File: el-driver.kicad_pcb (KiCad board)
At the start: 2 copper layers, 39 x 26 mm, 39 parts, among them J1 Conn_01x03, J2 Conn_01x02, Q1 SI3493DDV-T1-GE3, Q2 BSS138, Q3 BSS214NW, Q4 BSS214NW, T1 42XL003-RC, U1 NE555D

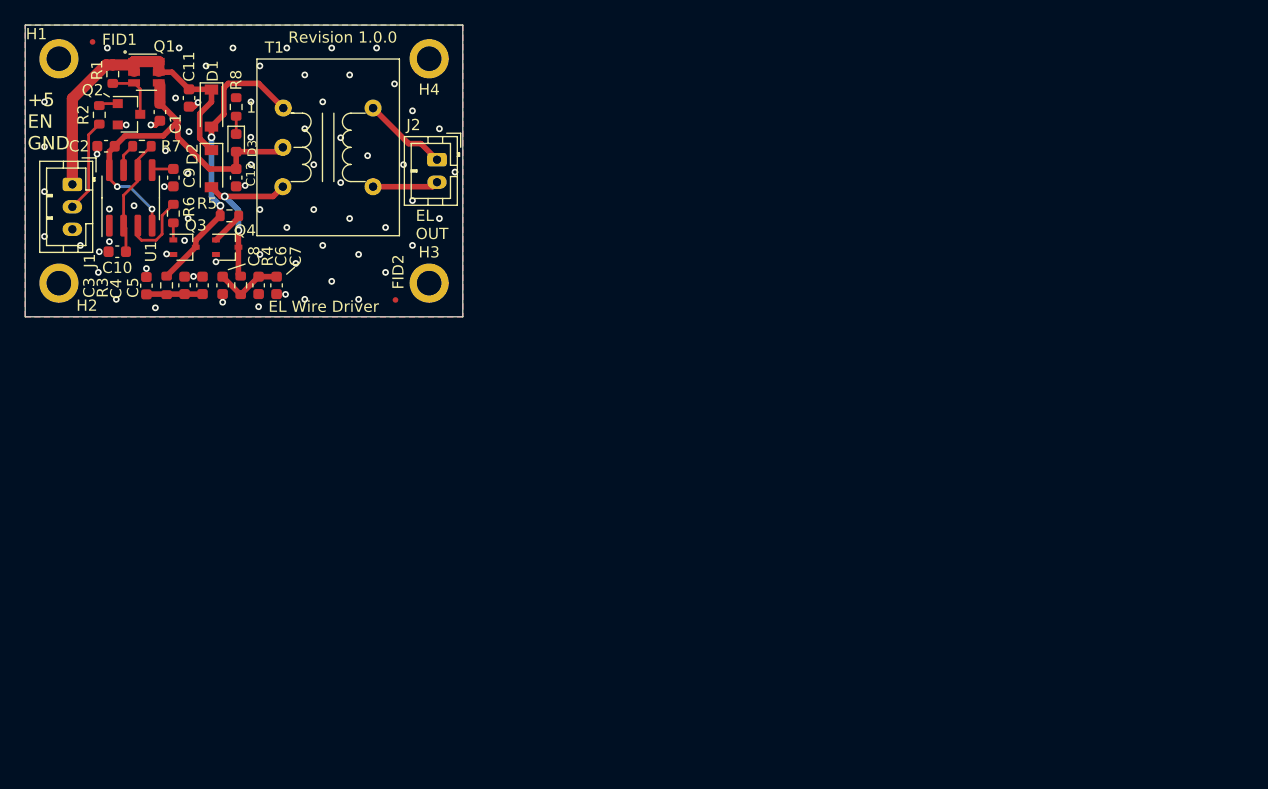
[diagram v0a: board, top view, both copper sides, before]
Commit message: Version 2.0.0
Signed-off-by: Aaron Williams <aaron.w2@gmail.com>
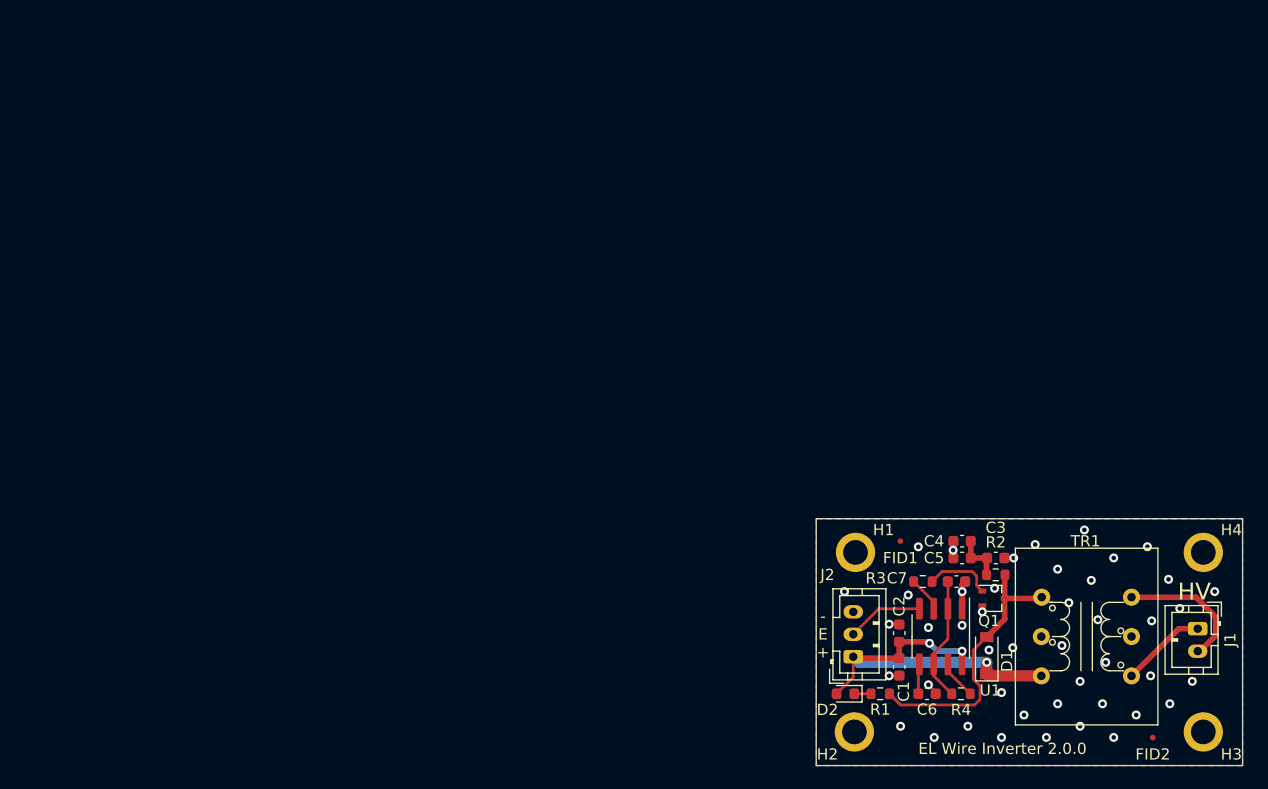
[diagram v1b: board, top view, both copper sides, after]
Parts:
- removed C10: 47nF, Capacitor_SMD:C_0603_1608Metric
- removed C11: 10uF, Capacitor_SMD:C_0603_1608Metric
- removed C12: 1uF, Capacitor_SMD:C_0603_1608Metric
- removed C8: 1nF, Capacitor_SMD:C_0603_1608Metric
- removed C9: 10nF, Capacitor_SMD:C_0603_1608Metric
- removed D3: LED, LED_SMD:LED_0603_1608Metric
- removed Q2: BSS138, Package_TO_SOT_SMD:SOT-23
- removed Q3, Q4: BSS214NW, Package_TO_SOT_SMD:SOT-323_SC-70
- removed R5, R6: 100k, Resistor_SMD:R_0603_1608Metric
- removed R7: 10k, Resistor_SMD:R_0603_1608Metric
- removed R8: 220, Resistor_SMD:R_0603_1608Metric
- removed the REF** at (114.3, 48.5)
- removed T1: 42XL003-RC, Aaron:Transformer_42XL_EI-14
- added REF**: OSHW-Logo2_7.3x6mm_SilkScreen, Symbol:OSHW-Logo2_7.3x6mm_SilkScreen, B.Cu at (194.1, 96.8)
- added TR1: Transformer-EI14, Aaron:Transformer_42XL_EI-14, F.Cu at (194.6, 88.5)
- C6: value 4.7nF -> 10nF
- C7: value 1nF -> 47nF
- D2: value SS24FL -> LED; footprint Diode_SMD:D_SOD-123 -> LED_SMD:LED_0603_1608Metric
- J1: value Conn_01x03 -> Conn_01x02; footprint Connector_JST:JST_PH_B3B-PH-K_1x03_P2.00mm_Vertical -> Connector_JST:JST_PH_B2B-PH-K_1x02_P2.00mm_Vertical
- J2: value Conn_01x02 -> Conn_01x03; footprint Connector_JST:JST_PH_B2B-PH-K_1x02_P2.00mm_Vertical -> Connector_JST:JST_PH_B3B-PH-K_1x03_P2.00mm_Vertical
- Q1: value SI3493DDV-T1-GE3 -> BSS214NW; footprint Package_TO_SOT_SMD:SOT-23-6 -> Package_TO_SOT_SMD:SOT-323_SC-70
- R1: value 100k -> 220
- R2: value 100k -> 39.2
- R3: value 39.2 -> 100k
- R4: value 39.2 -> 10k
- moved J1 107.8 mm to (204.5, 87.8)
- moved R2 89.8 mm to (186.5, 83.0), turned to 180 degrees
- moved Q1 88.9 mm to (186.3, 85.1)
- moved R1 87.9 mm to (176.2, 93.6), turned to 0 degrees
- moved REF** 87.3 mm to (182.4, 96.1)
- moved FID1 84.6 mm to (178.0, 80.0), turned to 180 degrees
- moved D1 84.6 mm to (185.7, 90.2), turned to 90 degrees
- moved H1 83.5 mm to (174.0, 81.0), turned to 180 degrees
- moved C2 83.0 mm to (177.9, 88.2), turned to 90 degrees
- moved C1 82.4 mm to (177.9, 91.2)
- moved U1 82.1 mm to (181.6, 88.5), turned to 270 degrees
- moved H4 81.8 mm to (205.0, 81.0), turned to 180 degrees
- moved H2 81.4 mm to (173.9, 97.0), turned to 180 degrees
- moved H3 79.8 mm to (205.0, 97.0), turned to 180 degrees
- moved C3 79.5 mm to (186.5, 81.5), turned to 0 degrees
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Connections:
- C1 pad 1: /5V_SW -> +5V
- C2 pad 1: /5V_SW -> +5V
- C7 pad 1: Net-(C6-Pad1) -> Net-(C7-Pad1)
- D2 pad 1: +5V -> Net-(D2-Pad1)
- D2 pad 2: Net-(D2-Pad2) -> +5V
- J1 pad 1: +5V -> Net-(J1-Pad1)
- J1 pad 2: /EN -> Net-(J1-Pad2)
- J2 pad 1: Net-(J2-Pad1) -> +5V
- J2 pad 2: Net-(J2-Pad2) -> /EN
- Q1 pad 1: +5V -> Net-(Q1-Pad1)
- Q1 pad 2: +5V -> GND
- Q1 pad 3: Net-(Q1-Pad3) -> Net-(D1-Pad2)
- R1 pad 1: +5V -> Net-(D2-Pad1)
- R1 pad 2: Net-(Q1-Pad3) -> Net-(D1-Pad2)
- R2 pad 1: /EN -> Net-(D1-Pad2)
- R2 pad 2: Net-(Q2-Pad1) -> Net-(C3-Pad1)
- R3 pad 1: Net-(D1-Pad2) -> Net-(R3-Pad1)
- R3 pad 2: Net-(C3-Pad1) -> Net-(Q1-Pad1)
- R4 pad 1: Net-(D2-Pad2) -> Net-(R4-Pad1)
- R4 pad 2: Net-(C6-Pad1) -> Net-(C7-Pad1)
- U1 pad 2: Net-(C10-Pad1) -> Net-(C7-Pad1)
- U1 pad 3: Net-(R6-Pad1) -> Net-(R3-Pad1)
- U1 pad 4: /5V_SW -> /EN
- U1 pad 5: Net-(C9-Pad1) -> Net-(C6-Pad1)
- U1 pad 6: Net-(C10-Pad1) -> Net-(C7-Pad1)
- U1 pad 7: Net-(R7-Pad1) -> Net-(R4-Pad1)
- U1 pad 8: /5V_SW -> +5V
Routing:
- net /5V_SW: track 33.6 -> 0.00 mm, vias 2 -> 0
- net Net-(D2-Pad2): track 14.8 -> 0.00 mm, vias 2 -> 0
- net Net-(J1-Pad2): track 0.00 -> 12.1 mm
- net Net-(C7-Pad1): track 0.00 -> 11.2 mm
- net Net-(C10-Pad1): track 10.5 -> 0.00 mm
- net Net-(J1-Pad1): track 0.00 -> 7.64 mm
- net Net-(J2-Pad1): track 7.61 -> 0.00 mm
- net Net-(R6-Pad1): track 6.57 -> 0.00 mm
- net Net-(Q1-Pad1): track 0.00 -> 6.07 mm
- net Net-(J2-Pad2): track 5.87 -> 0.00 mm
- net Net-(Q1-Pad3): track 4.95 -> 0.00 mm
- net +5V: track 30.1 -> 34.7 mm, vias 0 -> 3
- net Net-(C6-Pad1): track 6.14 -> 2.66 mm
- net Net-(R4-Pad1): track 0.00 -> 3.45 mm
- net Net-(R3-Pad1): track 0.00 -> 3.17 mm
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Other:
- board size 39 x 26 mm -> 38 x 22 mm
- board text added: "- E +"
- board text added: "EL Wire Inverter 2.0.0"
- board text added: "G EN +5"
- board text added: "HV"
- board text removed: "+5 +Enable GND"
- board text removed: "+5 EN GND"
- board text removed: "EL OUT"
- board text removed: "EL Wire Driver"
- board text removed: "Revision 1.0.0"
- board text removed: "To enable, apply +5V to EN."
